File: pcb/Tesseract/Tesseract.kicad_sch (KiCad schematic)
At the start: 23 parts, among them IC1 MAX98357AETE+T, J1 NHD-1.91-176176UBC3 Conn-1, J2 USB C Power Connector, J3 Speaker Connector, J4 RPI Power Connector, J5 LED Strip Connector, J6 RPI Signal Connector 1, J7 RPI Signal Connector 2, J8 NHD-1.91-176176UBC3 Conn-2, SW1 SW_Push, SW2 SW_Push, SW3 SW_Push, SW4 SW_Push

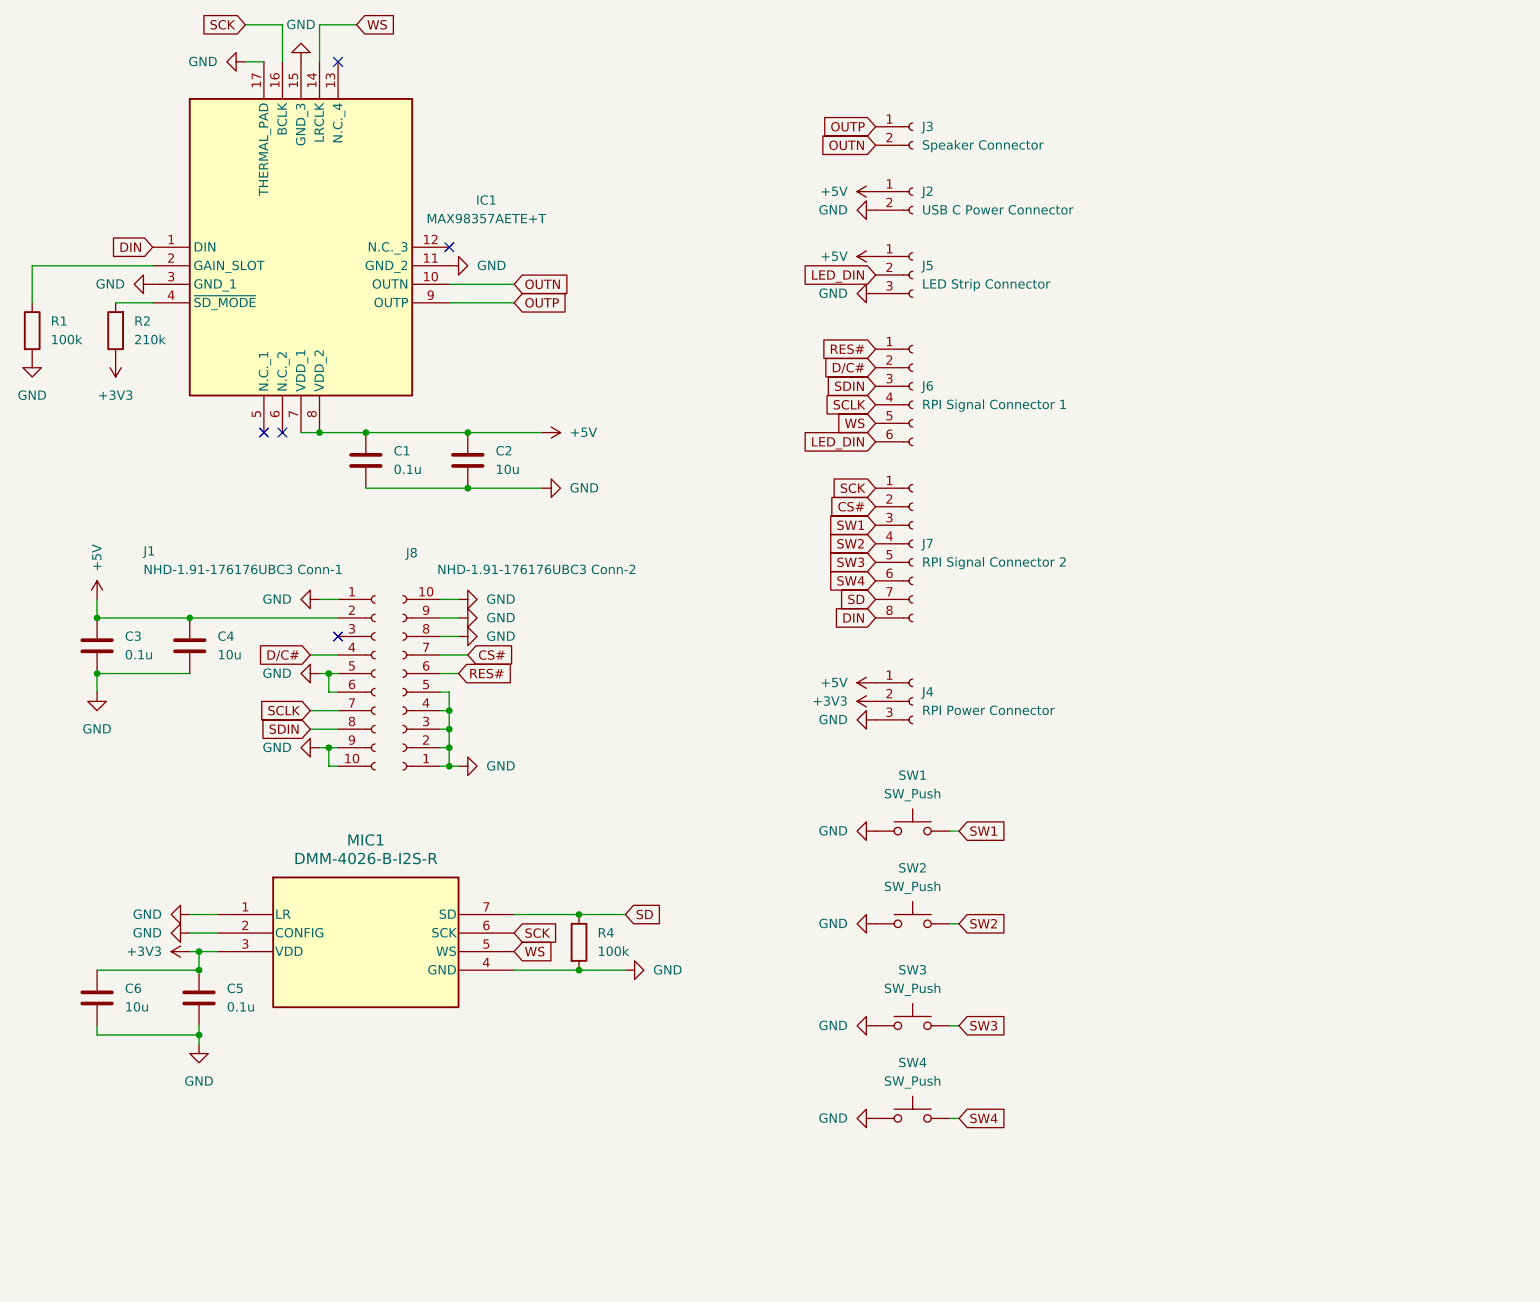
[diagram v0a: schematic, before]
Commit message: Update PCB and schematic related files
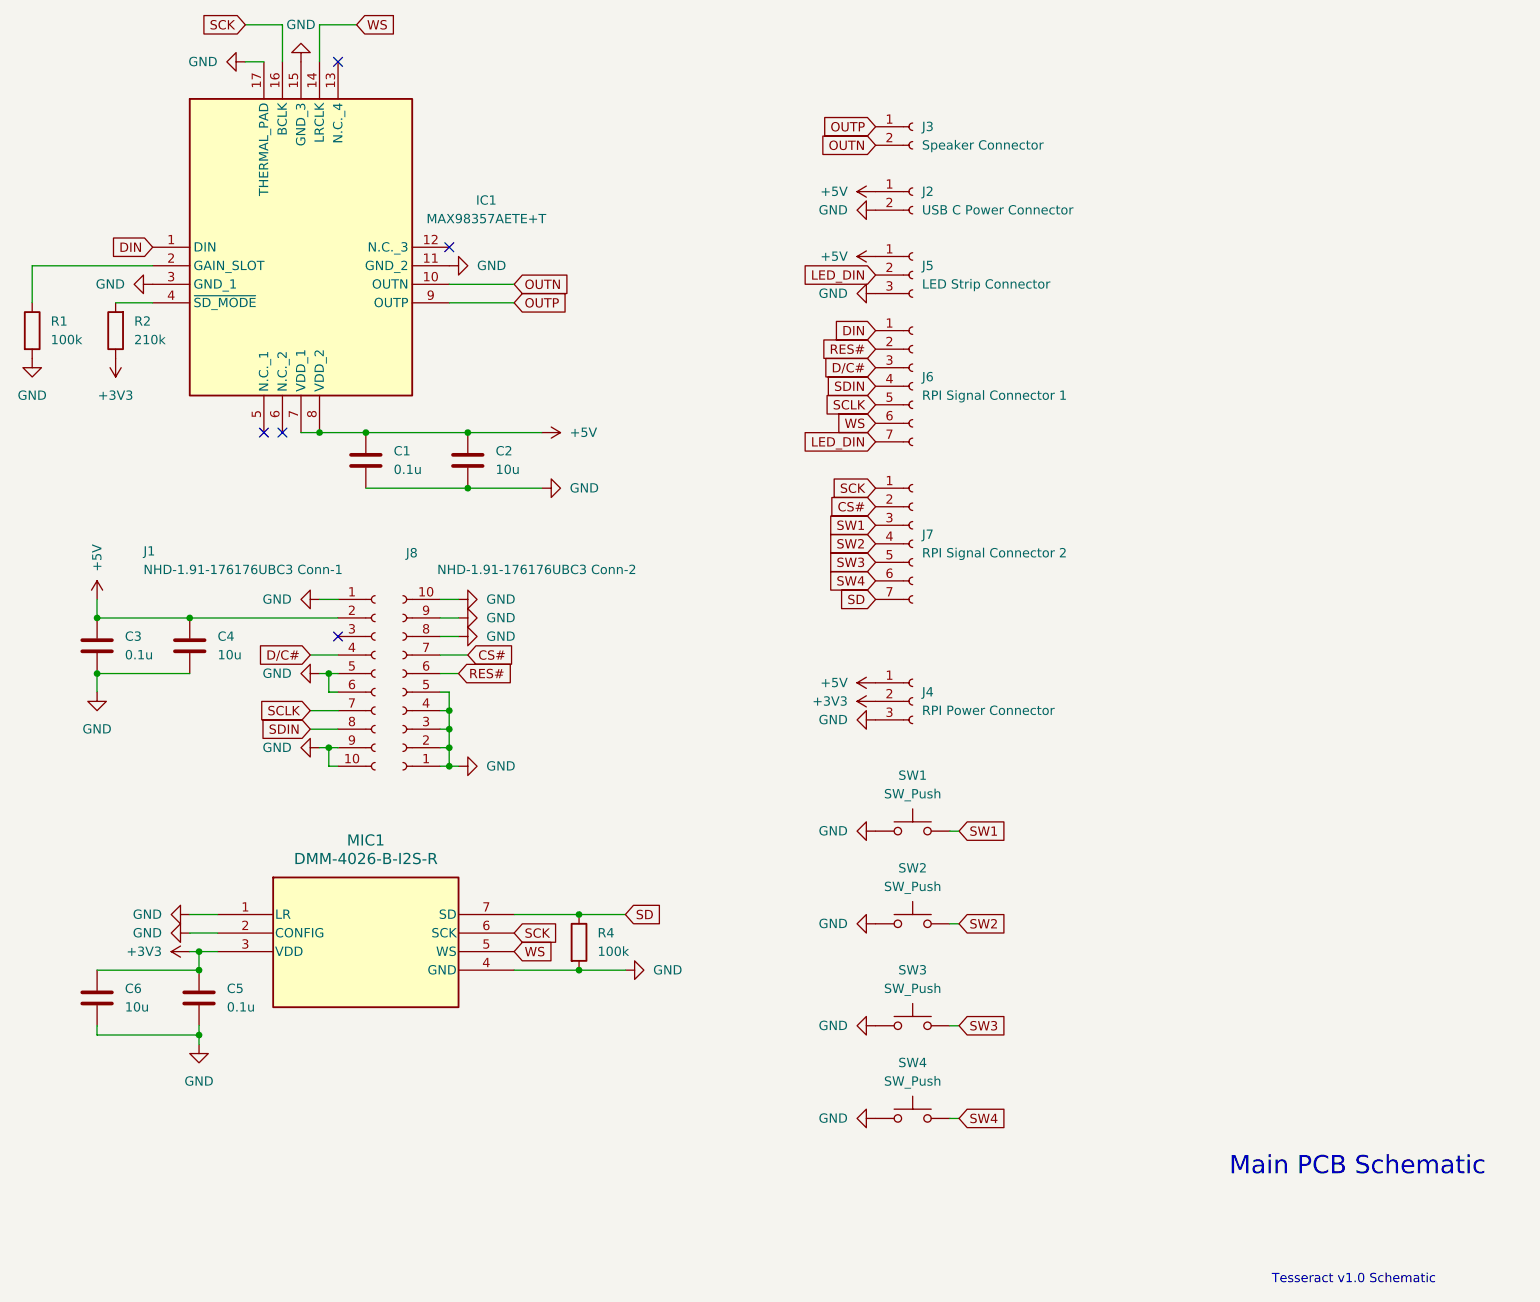
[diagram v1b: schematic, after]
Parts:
- J6: footprint Connector_JST:JST_XH_B6B-XH-A_1x06_P2.50mm_Vertical -> Connector_JST:JST_XH_B7B-XH-A_1x07_P2.50mm_Vertical; symbol Connector:Conn_01x06_Socket -> Connector:Conn_01x07_Socket
- J7: footprint Connector_JST:JST_XH_B8B-XH-A_1x08_P2.50mm_Vertical -> Connector_JST:JST_XH_B7B-XH-A_1x07_P2.50mm_Vertical; symbol Connector:Conn_01x08_Socket -> Connector:Conn_01x07_Socket
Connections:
- net DIN: now also J6.1 (Pin_1); no longer J7.8 (Pin_8)
- net D/C#: now also J6.3 (Pin_3); no longer J6.2 (Pin_2)
- net LED_DIN: now also J6.7 (Pin_7); no longer J6.6 (Pin_6)
- net RES#: now also J6.2 (Pin_2); no longer J6.1 (Pin_1)
- net SCLK: now also J6.5 (Pin_5); no longer J6.4 (Pin_4)
- net SDIN: now also J6.4 (Pin_4); no longer J6.3 (Pin_3)
- net WS: now also J6.6 (Pin_6); no longer J6.5 (Pin_5)
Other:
- note added: "Main PCB Schematic"
- note added: "Tesseract v1.0 Schematic"
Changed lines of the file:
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@@
 	(generator_version "9.0")
 	(paper "A4")
+	(text "Main PCB Schematic"
+		(exclude_from_sim no)
+		(at 199.39 174.244 0)
+		(effects
+			(font
+				(size 2.5 2.5)
+				(thickness 0.3125)
+				(color 0 0 0 1)
+			)
+		)
+	)
+	(text "Tesseract v1.0 Schematic"
+		(exclude_from_sim no)
+		(at 198.882 189.738 0)
+		(effects
+			(font
+				(size 1.27 1.27)
+			)
+		)
+	)
 	(junction
 		(at 40.64 144.78)
@@
 	(global_label "DIN"
 		(shape input)
-		(at 133.35 99.06 180)
+		(at 133.35 59.69 180)
 		(fields_autoplaced yes)
 		(effects
@@
 		)
 		(property "Intersheetrefs" "${INTERSHEET_REFS}"
-			(at 127.1595 99.06 0)
+			(at 127.1595 59.69 0)
 			(effects
 				(font
@@
 	)
 	(symbol
-		(lib_id "Connector:Conn_01x08_Socket")
+		(lib_id "Connector:Conn_01x07_Socket")
 		(at 138.43 88.9 0)
 		(unit 1)
@@
 		(fields_autoplaced yes)
 		(property "Reference" "J7"
-			(at 139.7 88.8999 0)
+			(at 139.7 87.6299 0)
 			(effects
 				(font
@@
 		)
 		(property "Value" "RPI Signal Connector 2"
-			(at 139.7 91.4399 0)
+			(at 139.7 90.1699 0)
 			(effects
 				(font
@@
 			)
 		)
-		(property "Footprint" "Connector_JST:JST_XH_B8B-XH-A_1x08_P2.50mm_Vertical"
+		(property "Footprint" "Connector_JST:JST_XH_B7B-XH-A_1x07_P2.50mm_Vertical"
 			(at 138.43 88.9 0)
 			(effects
@@
 			)
 		)
-		(property "Description" "Generic connector, single row, 01x08, script generated"
+		(property "Description" "Generic connector, single row, 01x07, script generated"
 			(at 138.43 88.9 0)
 			(effects
@@
 		(pin "7"
 		)
-		(pin "8"
-		)
 		(pin "4"
 		)
@@
 	)
 	(symbol
-		(lib_id "Connector:Conn_01x06_Socket")
+		(lib_id "Connector:Conn_01x07_Socket")
 		(at 138.43 67.31 0)
 		(unit 1)
@@
 		(fields_autoplaced yes)
 		(property "Reference" "J6"
-			(at 139.7 67.3099 0)
+			(at 139.7 66.0399 0)
 			(effects
 				(font
@@
 		)
 		(property "Value" "RPI Signal Connector 1"
-			(at 139.7 69.8499 0)
+			(at 139.7 68.5799 0)
 			(effects
 				(font
@@
 			)
 		)
-		(property "Footprint" "Connector_JST:JST_XH_B6B-XH-A_1x06_P2.50mm_Vertical"
+		(property "Footprint" "Connector_JST:JST_XH_B7B-XH-A_1x07_P2.50mm_Vertical"
 			(at 138.43 67.31 0)
 			(effects
@@
 			)
 		)
-		(property "Description" "Generic connector, single row, 01x06, script generated"
+		(property "Description" "Generic connector, single row, 01x07, script generated"
 			(at 138.43 67.31 0)
 			(effects
@@
 		(pin "5"
 		)
+		(pin "7"
+		)
 		(instances
